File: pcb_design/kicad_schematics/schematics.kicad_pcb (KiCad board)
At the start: 2 copper layers, 57.5 x 33 mm, 29 parts, among them J11 BUTTON-HS-KEY1B, J6 PICKIT, J7 I2C_Communication_Protocol, J8 M22-2510205, J9 SG90, U1 PIC24FJ64GA702-I_SO, U2 ESP8266-01_ESP-01, U3 LM1117LD-3.3, Y2 16MHz crystal

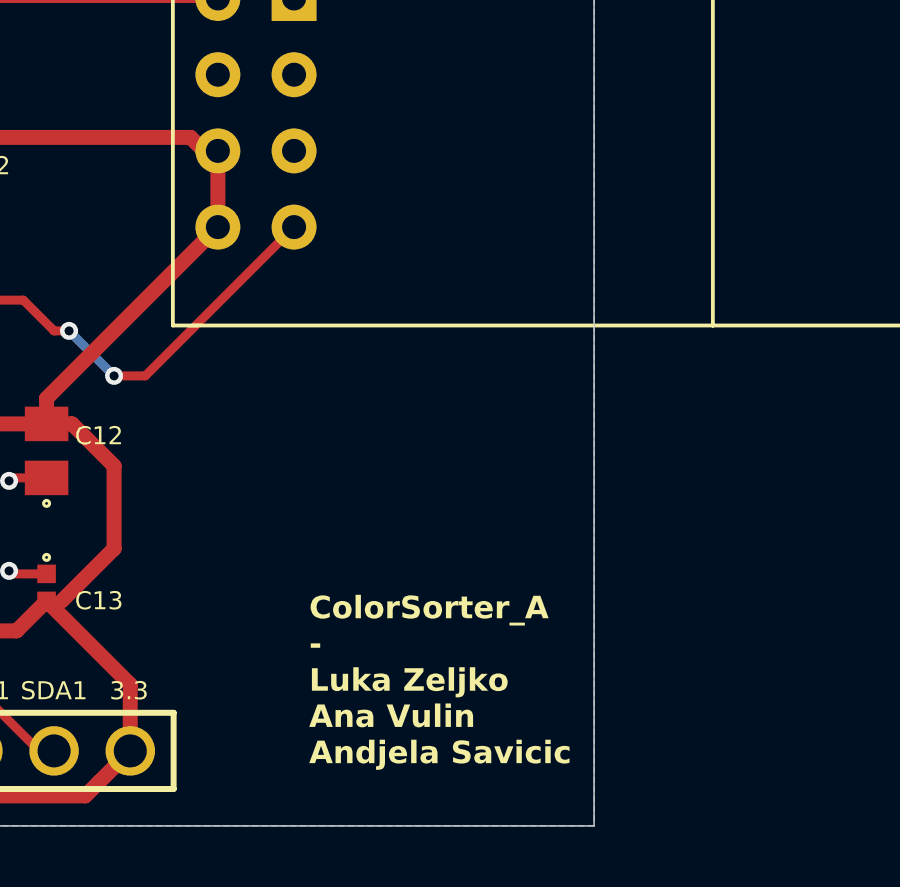
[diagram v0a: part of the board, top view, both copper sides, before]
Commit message: Povecan font imena inzenjera
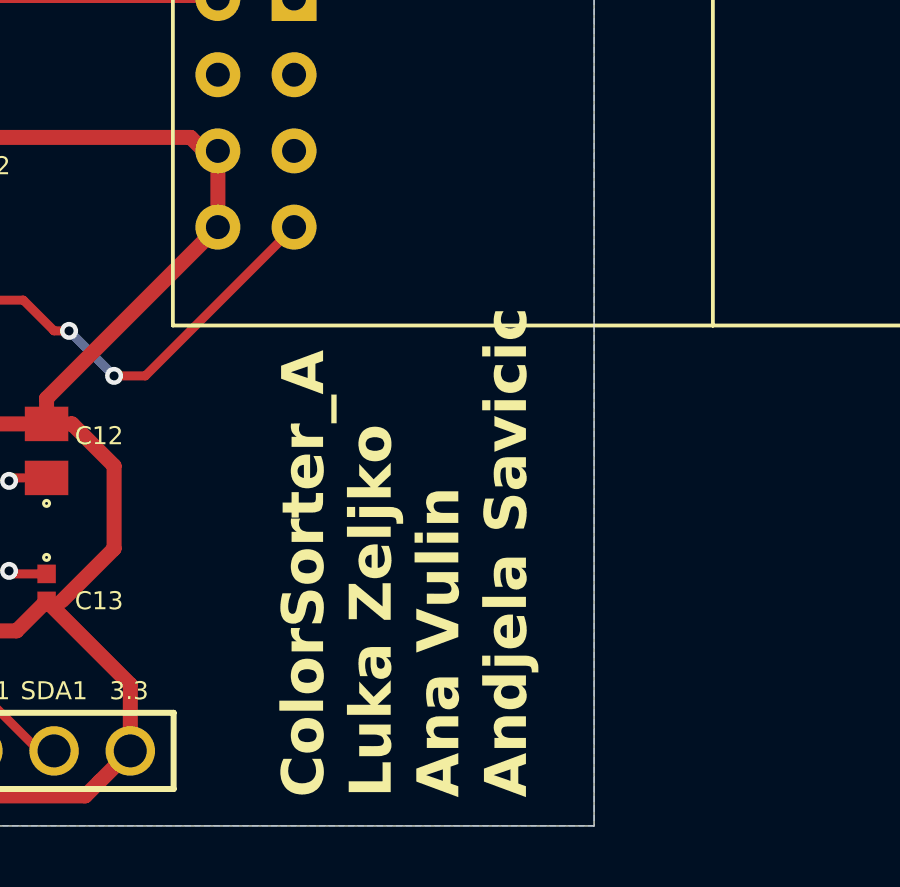
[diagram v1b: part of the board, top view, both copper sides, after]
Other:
- board text added: "ColorSorter_A Luka Zeljko Ana Vulin Andjela Savicic"
- board text removed: "ColorSorter_A - Luka Zeljko Ana Vulin Andjela Savicic"
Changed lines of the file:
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@@
 		)
 	)
-	(gr_text "ColorSorter_A\n-\nLuka Zeljko\nAna Vulin\nAndjela Savicic"
-		(at 165.5 79 0)
+	(gr_text "ColorSorter_A\nLuka Zeljko\nAna Vulin\nAndjela Savicic"
+		(at 172.9 80.05 90)
 		(layer "F.SilkS")
 		(effects
 			(font
-				(size 0.75 0.75)
-				(thickness 0.025)
+				(size 1.4 1.4)
+				(thickness 0.3)
 				(bold yes)
 			)
